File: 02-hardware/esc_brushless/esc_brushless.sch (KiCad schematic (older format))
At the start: 0 parts

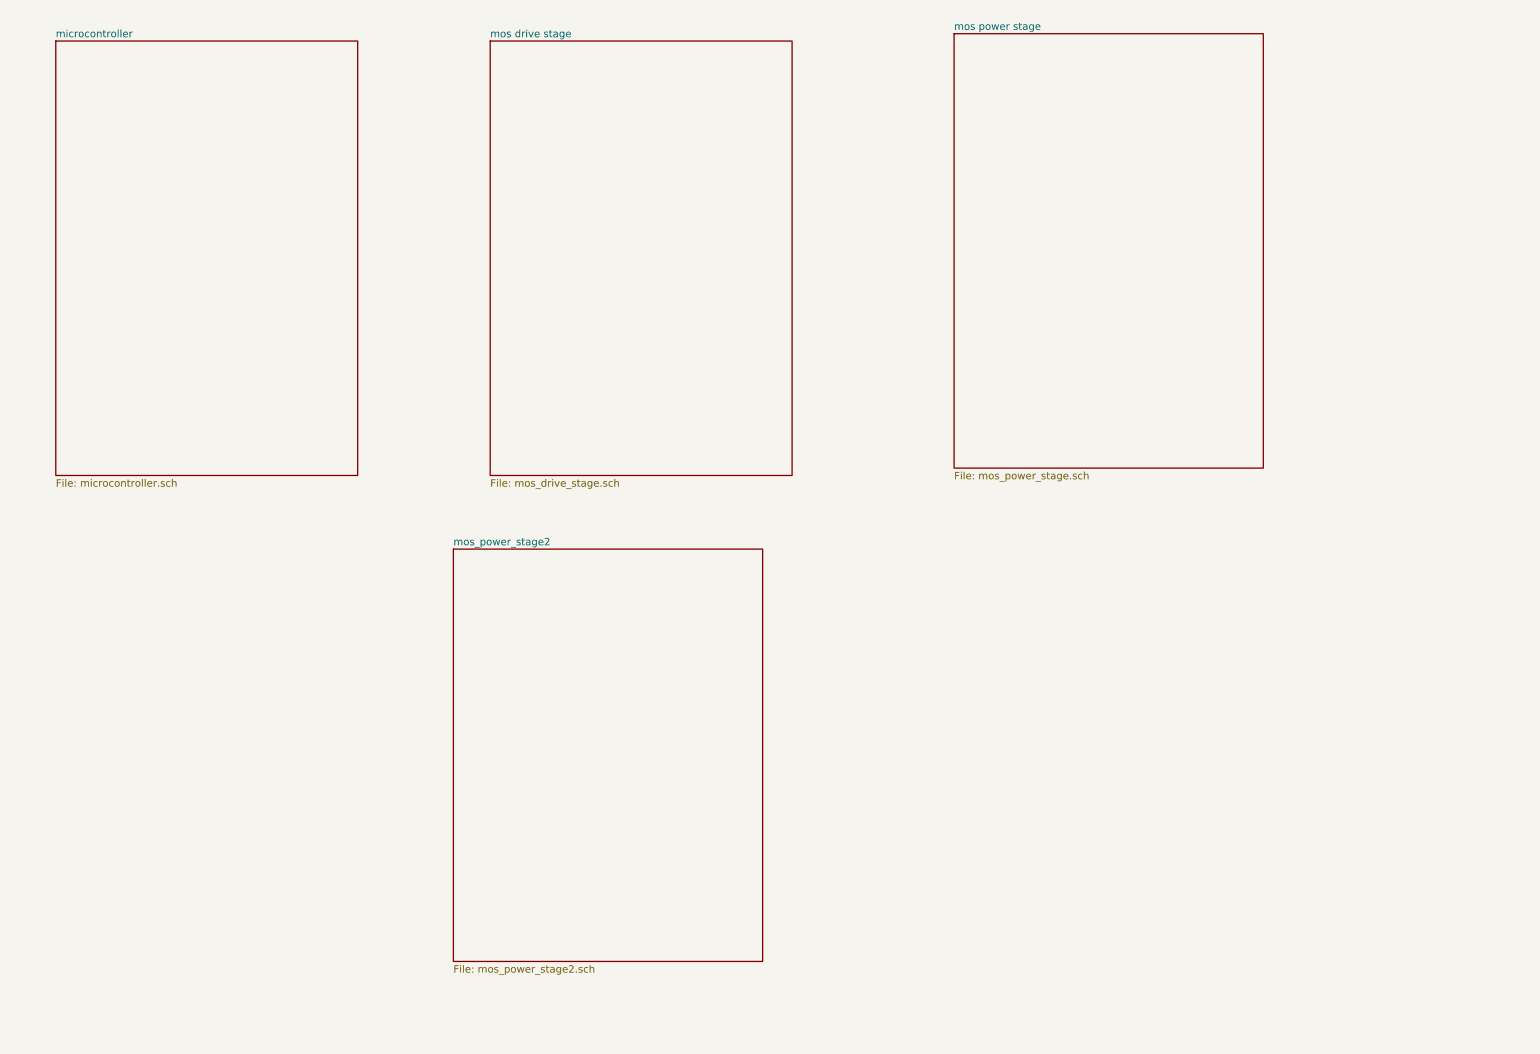
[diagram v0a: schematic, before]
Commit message: Schematics v1.0 - Architecture V1.0, fix DRC issues
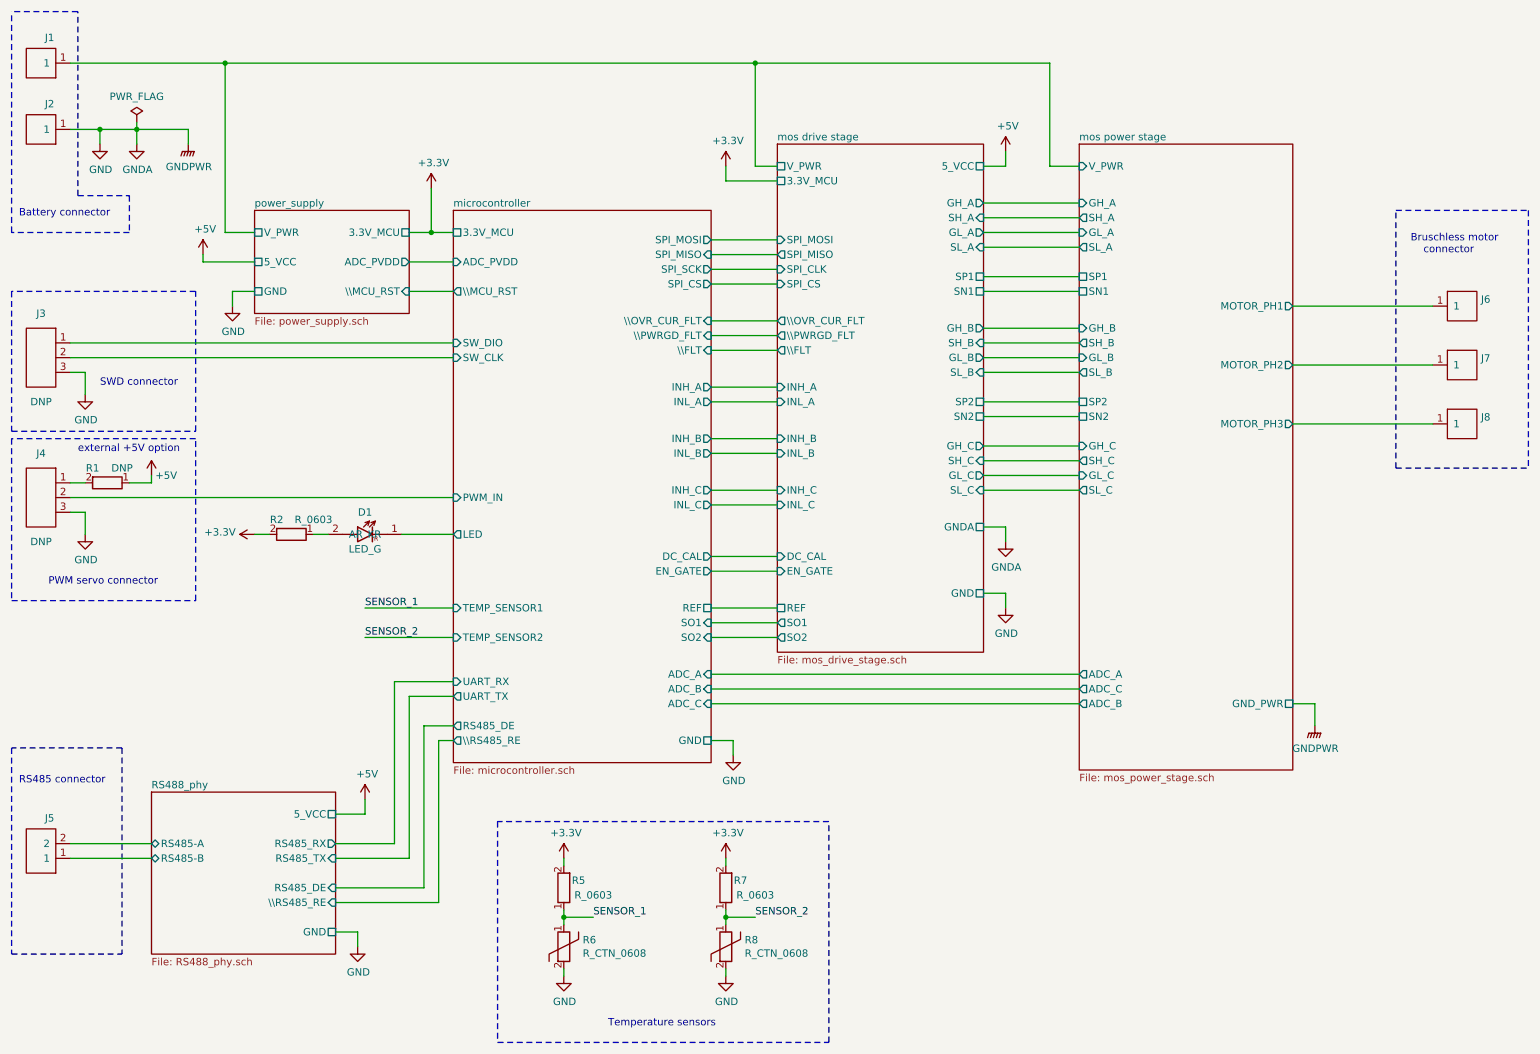
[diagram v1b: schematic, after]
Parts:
- added D1: LED_G, p_Package_Diode_SMD:LED_0603_1608Metric, symbol p_Diode:LED_G
- added J1, J2: Conn_HE13_1x1_5.08V, p_Package_Misc:PinHeader_1x01_P5.08mm_Vertical, symbol p_Misc:Conn_HE13_1x1_5.08V
- added J3, J4: DNP, p_Package_Misc:PinHeader_1x03_P2.54mm_Vertical, symbol esc_brushless-rescue:Conn_HE13_1x3_2.54-p_Misc
- added J5: Conn_HE13_1x2_2.54V, p_Package_Misc:PinHeader_1x02_P2.54mm_Vertical, symbol p_Misc:Conn_HE13_1x2_2.54V
- added J6, J7, J8: DNP, p_Package_Misc:PinHeader_1x01_P5.08mm_Vertical, symbol p_Misc:Conn_HE13_1x1_5.08V
- added R1: DNP, p_Package_Resistor_SMD:R_0603_1608Metric_Pad0.98x0.95mm_HandSolder, symbol p_Passive:R_0603
- added R2, R5, R7: R_0603, p_Package_Resistor_SMD:R_0603_1608Metric_Pad0.98x0.95mm_HandSolder, symbol p_Passive:R_0603
- added R6, R8: R_CTN_0608, p_Package_Resistor_SMD:R_0603_1608Metric_Pad0.98x0.95mm_HandSolder, symbol p_Passive:R_CTN_0608
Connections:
- new net: J4.1, R1.2
- new net: D1.2 (AR), R2.1
- new net +3V3: R2.2, R5.2, R7.2
- new net +5V: R1.1
- new net GND: J2.1, J3.3, J4.3, R6.2, R8.2
- new net RS488_phy/RS485-A: J5.2
- new net RS488_phy/RS485-B: J5.1
- new net SENSOR_1: R5.1, R6.1
- new net SENSOR_2: R7.1, R8.1
- new net microcontroller/LED: D1.1 (KR)
- new net microcontroller/PWM_IN: J4.2
- new net microcontroller/SW_CLK: J3.2
- new net microcontroller/SW_DIO: J3.1
- new net mos drive stage/V_PWR: J1.1
- new net mos power stage/MOTOR_PH1: J6.1
- new net mos power stage/MOTOR_PH2: J7.1
- new net mos power stage/MOTOR_PH3: J8.1
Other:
- note added: "Battery connector"
- note added: "Bruschless motor\n connector"
- note added: "PWM servo connector"
- note added: "RS485 connector"
- note added: "SWD connector"
- note added: "Temperature sensors"
- note added: "external +5V option"
